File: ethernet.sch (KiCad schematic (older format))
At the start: 21 parts

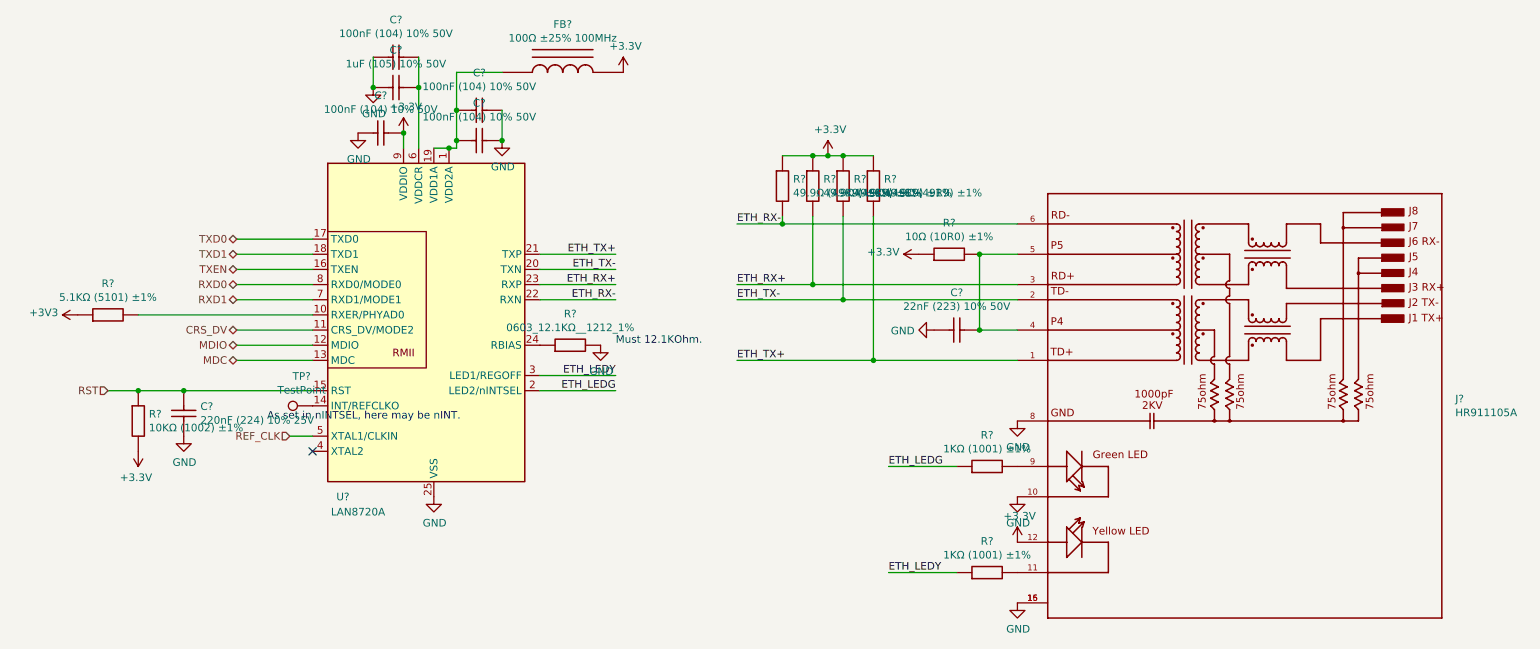
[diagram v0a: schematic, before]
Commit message: 20191113未完工
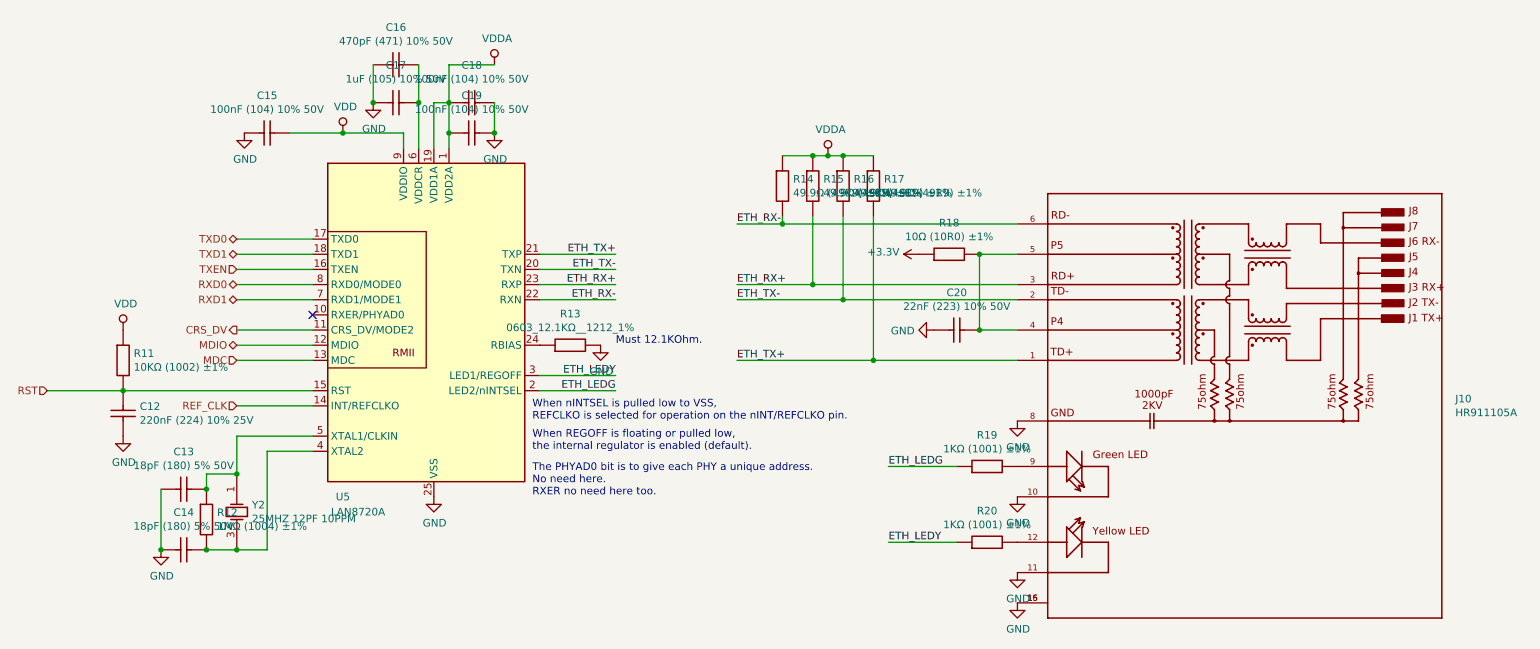
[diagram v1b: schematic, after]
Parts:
- removed C?: 0603_100nF__104_10%_50V, lc_lib:0603_C, symbol lc_Cap:0603_100nF__104_10%_50V
- removed FB?: 0805_100Ω_25%_100MHz, lc_lib:0805_L, symbol lc_IUD:0805_100Ω_25%_100MHz
- removed R?: 0603_5.1KΩ__5101_1%, lc_lib:0603_R, symbol lc_RES:0603_5.1KΩ__5101_1%
- removed TP?: TestPoint, symbol Connector:TestPoint
- added C13, C14: 0603_18pF__180_5%_50V, lc_lib:0603_C, symbol lc_Cap:0603_18pF__180_5%_50V
- added C16: 0603_470pF__471_10%_50V, lc_lib:0603_C, symbol lc_Cap:0603_470pF__471_10%_50V
- added R12: 0603_1MΩ__1004_1%, lc_lib:0603_R, symbol lc_RES:0603_1MΩ__1004_1%
- added Y2: SMD-3225_4P__25MHZ_12PF_10PPM, lc_lib:SMD-3225_4P, symbol lc_CrystalOscillator:SMD-3225_4P__25MHZ_12PF_10PPM
- gave numbers to parts that had none: 17
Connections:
- net +3V3: no longer C15.2, J10.12 (YA), R11.2, R14.1, R15.1, R16.1, R17.1, U5.9 (VDDIO)
- net GND: now also J10.11 (YC), C13.1, C14.1, C16.1
- net REF_CLK: now also U5.14 (INT/REFCLKO); no longer U5.5 (XTAL1/CLKIN)
- net RST: now also R11.2; no longer R11.1
- net VDDA: now reaches C18.1, C19.1, U5.1 (VDD2A), U5.19 (VDD1A)
- net VDDA: now also R14.1, R15.1, R16.1, R17.1
- net at U5.4 (XTAL2): now also C14.2, R12.2, Y2.3 (OSC2)
- net at C17.2, U5.6 (VDDCR): now also C16.2
- net at R20.2: now also J10.12 (YA); no longer J10.11 (YC)
- new net: C13.2, R12.1, U5.5 (XTAL1/CLKIN), Y2.1 (OSC1)
- new net VDD: C15.2, R11.1, U5.9 (VDDIO)
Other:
- note added: "The PHYAD0 bit is to give each PHY a unique address.\nNo need here.\nRXER no need here too."
- note added: "When REGOFF is floating or pulled low, \nthe internal regulator is enabled (default).\n"
- note added: "When nINTSEL is pulled low to VSS, \nREFCLKO is selected for operation on the nINT/REFCLKO pin."
- note removed: "As set in nINTSEL, here may be nINT."
- moved on the sheet: C12, C15, C17, C18, C19, R11, R20
